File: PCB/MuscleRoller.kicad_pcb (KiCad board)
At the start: 2 copper layers, 66 x 64 mm, 28 parts, among them J1 Screw_Terminal_01x02, J10 Conn_01x04_Male, J11 Conn_01x03_Male, J12 Conn_01x03_Male, J2 Conn_02x03_Odd_Even, J3 Conn_02x03_Odd_Even, J4 Conn_01x04_Male, J5 Conn_01x04_Male, J6 Conn_01x03_Male, J7 Conn_01x04_Male, J8 Conn_01x04_Male, J9 Conn_01x04_Male, U1 AZ1117-3.3, U2 ESP32-S2-WROOM

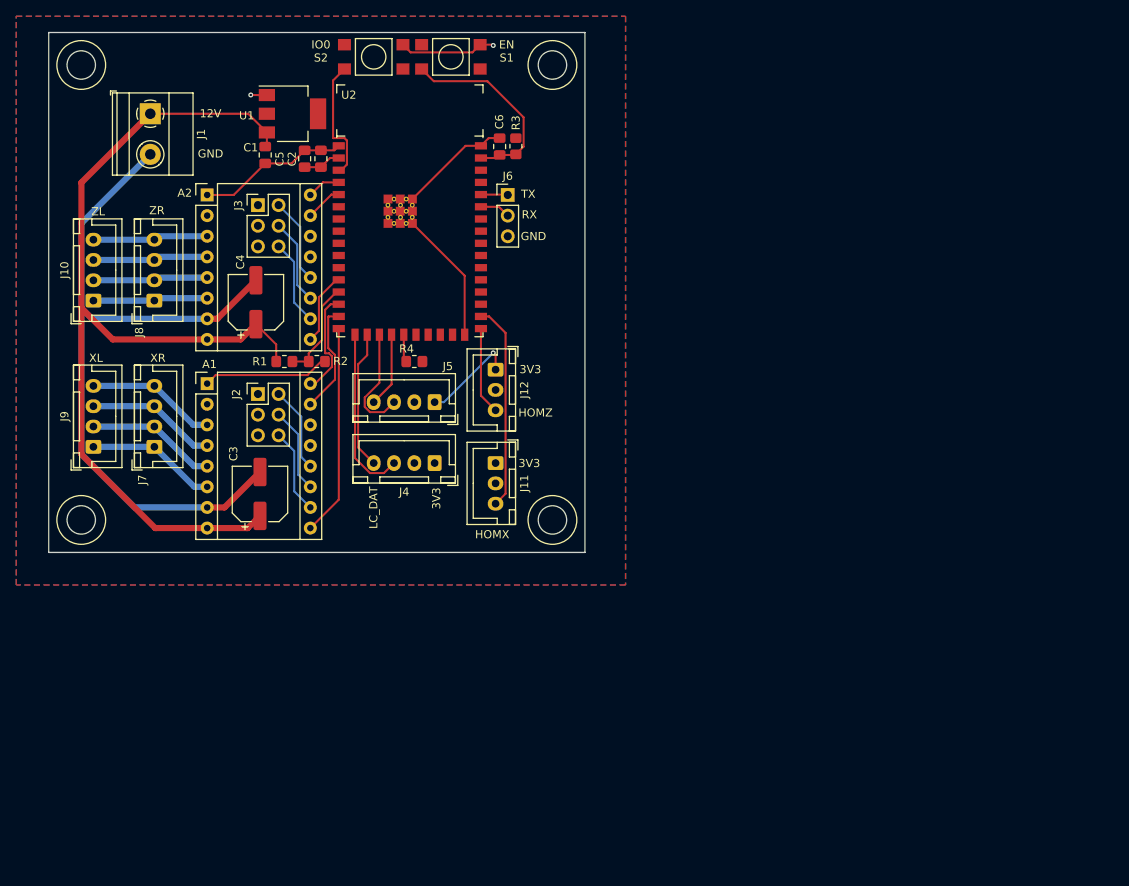
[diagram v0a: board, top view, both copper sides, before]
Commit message: PCB complete
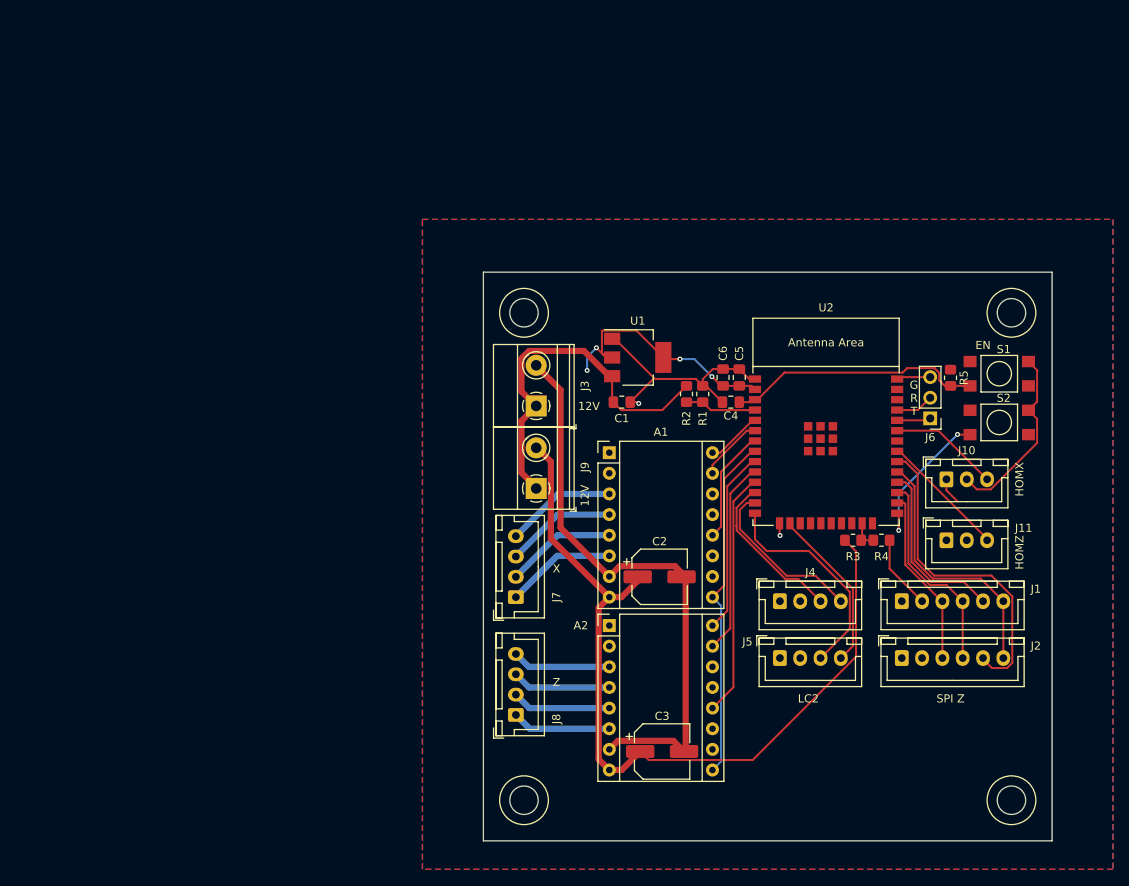
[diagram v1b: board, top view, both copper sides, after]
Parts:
- removed J12: Conn_01x03_Male, Connector_JST:JST_XH_B3B-XH-A_1x03_P2.50mm_Vertical
- added R5: 10K, Resistor_SMD:R_0805_2012Metric_Pad1.20x1.40mm_HandSolder, F.Cu at (165.0, 94.5)
- C2: value 22u -> 100u; footprint Capacitor_SMD:C_0805_2012Metric_Pad1.18x1.45mm_HandSolder -> Capacitor_SMD:CP_Elec_6.3x7.7
- C4: value 100u -> 1u; footprint Capacitor_SMD:CP_Elec_6.3x7.7 -> Capacitor_SMD:C_0805_2012Metric_Pad1.18x1.45mm_HandSolder
- C5: value 0.1u -> 22U
- C6: value 1u -> 0.1u
- J1: value Screw_Terminal_01x02 -> Conn_01x06_Male; footprint TerminalBlock_Phoenix:TerminalBlock_Phoenix_MKDS-1,5-2_1x02_P5.00mm_Horizontal -> Connector_JST:JST_XH_B6B-XH-A_1x06_P2.50mm_Vertical
- J10: value Conn_01x04_Male -> Conn_01x03_Male; footprint Connector_JST:JST_XH_B4B-XH-A_1x04_P2.50mm_Vertical -> Connector_JST:JST_XH_B3B-XH-A_1x03_P2.50mm_Vertical
- J2: value Conn_02x03_Odd_Even -> Conn_01x06_Male; footprint Connector_PinHeader_2.54mm:PinHeader_2x03_P2.54mm_Vertical -> Connector_JST:JST_XH_B6B-XH-A_1x06_P2.50mm_Vertical
- J3: value Conn_02x03_Odd_Even -> Screw_Terminal_01x02; footprint Connector_PinHeader_2.54mm:PinHeader_2x03_P2.54mm_Vertical -> TerminalBlock_Phoenix:TerminalBlock_Phoenix_MKDS-1,5-2_1x02_P5.00mm_Horizontal
- J9: value Conn_01x04_Male -> Screw_Terminal_01x02; footprint Connector_JST:JST_XH_B4B-XH-A_1x04_P2.50mm_Vertical -> TerminalBlock_Phoenix:TerminalBlock_Phoenix_MKDS-1,5-2_1x02_P5.00mm_Horizontal
- R3: value 10K -> 47k
- U2: value ESP32-S2-WROOM -> ESP32-WROOM-E; footprint A4:ESP32-S2-WROOM -> Espressif:ESP32-WROOM-32E
- moved J1 110.3 mm to (159.0, 122.0), turned to 0 degrees
- moved J10 107.3 mm to (164.5, 107.0), turned to 0 degrees
- moved S2 89.2 mm to (171.0, 100.0)
- moved J2 85.7 mm to (159.0, 129.0)
- moved S1 78.0 mm to (171.0, 94.0)
- moved A2 72.5 mm to (123.0, 125.0)
- moved J8 67.7 mm to (111.5, 136.0)
- moved C2 66.2 mm to (129.2, 119.0), turned to 0 degrees
- moved R3 63.8 mm to (153.0, 114.5), turned to 0 degrees
- moved R4 61.6 mm to (156.5, 114.5), turned to 0 degrees
- moved C5 59.9 mm to (139.0, 94.5)
- moved C4 59.7 mm to (138.0, 97.5), turned to 180 degrees
- moved J6 58.8 mm to (162.5, 99.5), turned to 180 degrees
- moved C3 58.8 mm to (129.5, 140.5), turned to 0 degrees
- moved U2 58.2 mm to (149.7, 101.7)
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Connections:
- A1 pad 12: Net-(A1-Pad12) -> MSX
- A1 pad 8: +12V -> ESTOP12V
- A1 pad 9: ENX -> EN_STEP
- A2 pad 12: Net-(A2-Pad12) -> MSZ
- A2 pad 8: +12V -> ESTOP12V
- A2 pad 9: ENZ -> EN_STEP
- C2 pad 1: +3V3 -> ESTOP12V
- C3 pad 1: +12V -> ESTOP12V
- C4 pad 1: +12V -> EN
- C6 pad 1: EN -> +3V3
- J1 pad 1: +12V -> +3V3
- J10 pad 1: ZB2 -> +3V3
- J10 pad 2: ZB1 -> GND
- J10 pad 3: ZA1 -> HOMX
- J11 pad 3: HOMX -> HOMZ
- J2 pad 2: Net-(A1-Pad12) -> GND
- J2 pad 3: +3V3 -> CLK
- J2 pad 4: Net-(A1-Pad11) -> MISO
- J2 pad 5: +3V3 -> CS1
- J2 pad 6: Net-(A1-Pad10) -> MOSI
- J3 pad 1: +3V3 -> +12V
- J3 pad 2: Net-(A2-Pad12) -> GND
- J9 pad 1: XB2 -> +12V
- J9 pad 2: XB1 -> ESTOP12V
- R3 pad 1: +3V3 -> ESTOP12V
- R3 pad 2: EN -> ESTOP
- R4 pad 1: +3V3 -> ESTOP
- R4 pad 2: DAC2 -> GND
- U2 pad 10: Net-(U2-Pad10) -> STEPZ
- U2 pad 11: Net-(U2-Pad11) -> MSZ
- U2 pad 12: ENZ -> LC_CLK
- U2 pad 13: CHARGE -> LC_DAT
- U2 pad 14: DIRX -> LC_CLK2
- U2 pad 15: STEPX -> GND
- U2 pad 16: ENX -> LC_DAT2
- U2 pad 17: LC_CLK -> Net-(U2-Pad17)
- U2 pad 18: LC_DAT -> Net-(U2-Pad18)
- U2 pad 19: LC_CLK2 -> Net-(U2-Pad19)
- U2 pad 20: LC_DAT2 -> Net-(U2-Pad20)
- U2 pad 21: DAC2 -> Net-(U2-Pad21)
- U2 pad 23: Net-(U2-Pad23) -> ESTOP
- U2 pad 25: Net-(U2-Pad25) -> IO0
- U2 pad 26: GND -> CLK
- U2 pad 27: HOMZ -> MISO
- U2 pad 28: HOMX -> CS0
- U2 pad 29: Net-(U2-Pad29) -> MOSI
- U2 pad 3: IO0 -> EN
- U2 pad 30: Net-(U2-Pad30) -> CS1
- U2 pad 31: Net-(U2-Pad31) -> HOMZ
- U2 pad 33: Net-(U2-Pad33) -> HOMX
- U2 pad 34: Net-(U2-Pad34) -> TX
- U2 pad 35: Net-(U2-Pad35) -> RX
- U2 pad 37: RX -> Net-(U2-Pad37)
- U2 pad 38: TX -> GND
- U2 pad 39: Net-(U2-Pad39) -> (no net)
- U2 pad 4: DIRZ -> CHARGE
- U2 pad 5: STEPZ -> DIRX
- U2 pad 6: Net-(U2-Pad6) -> STEPX
- U2 pad 7: Net-(U2-Pad7) -> MSX
- U2 pad 8: Net-(U2-Pad8) -> EN_STEP
- U2 pad 9: Net-(U2-Pad9) -> DIRZ
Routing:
- net ESTOP12V: track 0.00 -> 101.5 mm
- net +12V: track 118.4 -> 44.9 mm
- net GND: track 187.4 -> 140.1 mm
- net EN_STEP: track 0.00 -> 42.5 mm
- net CS1: track 0.00 -> 39.8 mm
- net MOSI: track 0.00 -> 32.0 mm
- net MSZ: track 0.00 -> 30.1 mm
- net ENX: track 26.0 -> 0.00 mm
- net MISO: track 0.00 -> 25.5 mm
- net CS0: track 0.00 -> 22.0 mm
- net CLK: track 0.00 -> 22.0 mm
- net STEPZ: track 4.57 -> 23.8 mm
- net DIRZ: track 4.14 -> 22.6 mm
- net +3V3: track 16.6 -> 34.3 mm, vias 1 -> 4
- net MSX: track 0.00 -> 14.0 mm
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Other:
- board size 66 x 64 mm -> 70 x 70 mm
- board text added: "G R T"
- board text added: "LC2"
- board text added: "SPI Z"
- board text added: "X"
- board text added: "Z"
- board text removed: "3V3"
- board text removed: "GND"
- board text removed: "IO0"
- board text removed: "LC_DAT"
- board text removed: "RX"
- board text removed: "TX"
- board text removed: "XL"
- board text removed: "XR"
- board text removed: "ZL"
- board text removed: "ZR"
